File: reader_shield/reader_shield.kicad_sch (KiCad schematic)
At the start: 0 parts

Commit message: Describe sheets
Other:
- company: (none) -> rwilliaise
- title: (none) -> reader00 Shield
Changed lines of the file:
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@@
 (kicad_sch (version 20230121) (generator eeschema)
-  (paper "A4")
+  (paper "USLetter")
+  (title_block
+    (title "reader00 Shield")
+    (rev "1")
+    (company "rwilliaise")
+  )
   (sheet (at 64.77 88.9) (size 50.8 40.64) (fields_autoplaced)
     (stroke (width 0.1524) (type solid))

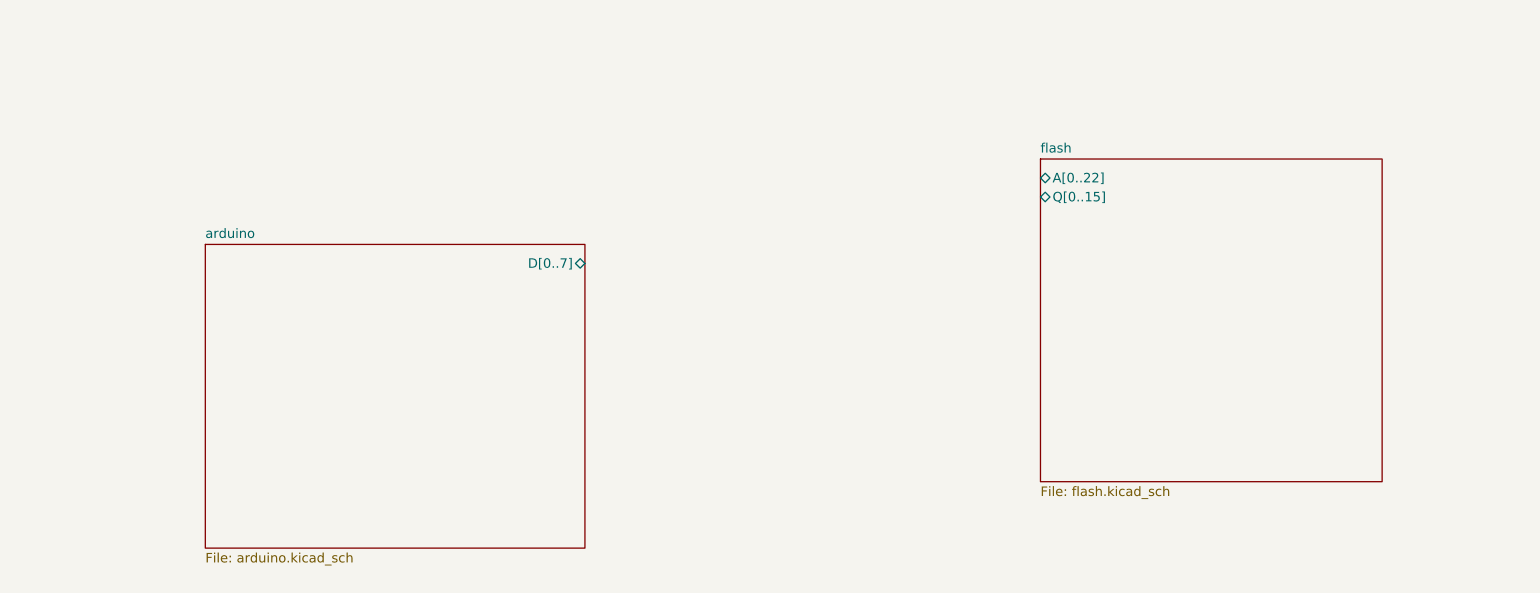
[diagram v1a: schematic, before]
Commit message: Revisions 1 and 2
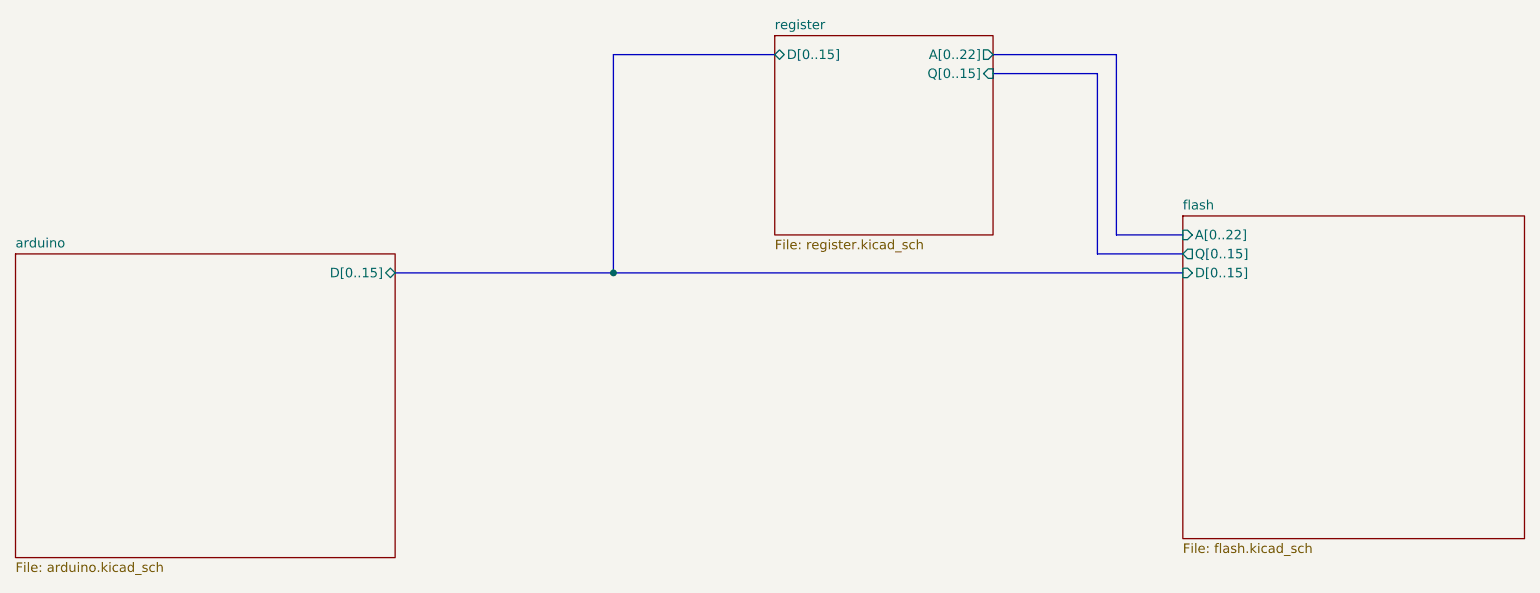
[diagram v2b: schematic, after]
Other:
- added sheet register (register.kicad_sch)
- sheet arduino ports: added D[0..15]; removed D[0..7]
- sheet flash ports: added D[0..15]; removed none
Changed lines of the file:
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@@
     (company "rwilliaise")
   )
-  (sheet (at 64.77 88.9) (size 50.8 40.64) (fields_autoplaced)
+  (junction (at 119.38 92.71) (diameter 0) (color 0 0 0 0)
+  )
+  (bus (pts (xy 170.18 63.5) (xy 186.69 63.5))
+    (stroke (width 0) (type default))
+  )
+  (bus (pts (xy 184.15 90.17) (xy 184.15 66.04))
+    (stroke (width 0) (type default))
+  )
+  (bus (pts (xy 90.17 92.71) (xy 119.38 92.71))
+    (stroke (width 0) (type default))
+  )
+  (bus (pts (xy 195.58 90.17) (xy 184.15 90.17))
+    (stroke (width 0) (type default))
+  )
+  (bus (pts (xy 119.38 92.71) (xy 195.58 92.71))
+    (stroke (width 0) (type default))
+  )
+  (bus (pts (xy 119.38 63.5) (xy 119.38 92.71))
+    (stroke (width 0) (type default))
+  )
+  (bus (pts (xy 186.69 87.63) (xy 195.58 87.63))
+    (stroke (width 0) (type default))
+  )
+  (bus (pts (xy 184.15 66.04) (xy 170.18 66.04))
+    (stroke (width 0) (type default))
+  )
+  (bus (pts (xy 119.38 63.5) (xy 140.97 63.5))
+    (stroke (width 0) (type default))
+  )
+  (bus (pts (xy 186.69 63.5) (xy 186.69 87.63))
+    (stroke (width 0) (type default))
+  )
+  (sheet (at 39.37 90.17) (size 50.8 40.64) (fields_autoplaced)
     (stroke (width 0.1524) (type solid))
     (fill (color 0 0 0 0.0000))
-    (property "Sheetname" "arduino" (at 64.77 88.1884 0)
+    (property "Sheetname" "arduino" (at 39.37 89.4584 0)
       (effects (font (size 1.27 1.27)) (justify left bottom))
     )
-    (property "Sheetfile" "arduino.kicad_sch" (at 64.77 130.1246 0)
+    (property "Sheetfile" "arduino.kicad_sch" (at 39.37 131.3946 0)
       (effects (font (size 1.27 1.27)) (justify left top))
     )
-    (pin "D[0..7]" bidirectional (at 115.57 91.44 0)
+    (pin "D[0..15]" bidirectional (at 90.17 92.71 0)
       (effects (font (size 1.27 1.27)) (justify right))
     )
@@
     )
   )
-  (sheet (at 176.53 77.47) (size 45.72 43.18) (fields_autoplaced)
+  (sheet (at 195.58 85.09) (size 45.72 43.18) (fields_autoplaced)
     (stroke (width 0.1524) (type solid))
     (fill (color 0 0 0 0.0000))
-    (property "Sheetname" "flash" (at 176.53 76.7584 0)
+    (property "Sheetname" "flash" (at 195.58 84.3784 0)
       (effects (font (size 1.27 1.27)) (justify left bottom))
     )
-    (property "Sheetfile" "flash.kicad_sch" (at 176.53 121.2346 0)
+    (property "Sheetfile" "flash.kicad_sch" (at 195.58 128.8546 0)
       (effects (font (size 1.27 1.27)) (justify left top))
     )
-    (pin "A[0..22]" bidirectional (at 176.53 80.01 180)
+    (pin "D[0..15]" input (at 195.58 92.71 180)
       (effects (font (size 1.27 1.27)) (justify left))
     )
-    (pin "Q[0..15]" bidirectional (at 176.53 82.55 180)
+    (pin "Q[0..15]" output (at 195.58 90.17 180)
+      (effects (font (size 1.27 1.27)) (justify left))
+    )
+    (pin "A[0..22]" input (at 195.58 87.63 180)
       (effects (font (size 1.27 1.27)) (justify left))
     )
@@
       )
     )
+  )
+  (sheet (at 140.97 60.96) (size 29.21 26.67) (fields_autoplaced)
+    (stroke (width 0.1524) (type solid))
+    (fill (color 0 0 0 0.0000))
+    (property "Sheetname" "register" (at 140.97 60.2484 0)
+      (effects (font (size 1.27 1.27)) (justify left bottom))
+    )
+    (property "Sheetfile" "register.kicad_sch" (at 140.97 88.2146 0)
+      (effects (font (size 1.27 1.27)) (justify left top))
+    )
+    (pin "A[0..22]" output (at 170.18 63.5 0)
+      (effects (font (size 1.27 1.27)) (justify right))
+    )
+    (pin "Q[0..15]" input (at 170.18 66.04 0)
+      (effects (font (size 1.27 1.27)) (justify right))
+    )
+    (pin "D[0..15]" bidirectional (at 140.97 63.5 180)
+      (effects (font (size 1.27 1.27)) (justify left))
+    )
+    (instances
+      (project "reader_shield"
+        (path "/6c6f8f01-73ee-4caa-8e4e-2be1e2e97b79" (page "4"))
+      )
+    )
